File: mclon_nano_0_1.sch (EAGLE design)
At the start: 69 parts, among them J2 10118194-0001LF/C, T1 2N2222, T1.1 BC847, T2 2N2222, T2.1 BC847, U1 TP5400, X1 AK550/2, X2 AK550/2, X3 AK550/2

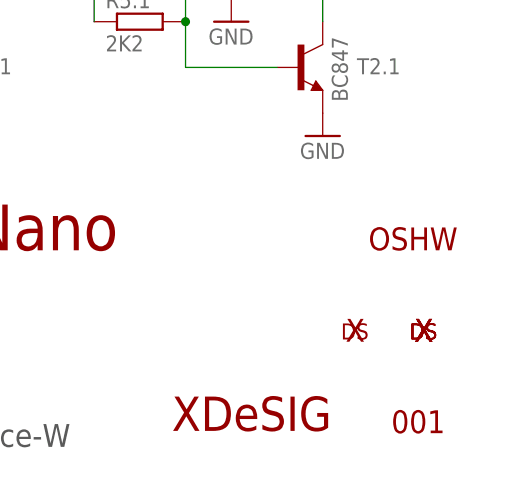
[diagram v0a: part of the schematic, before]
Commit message: Update img
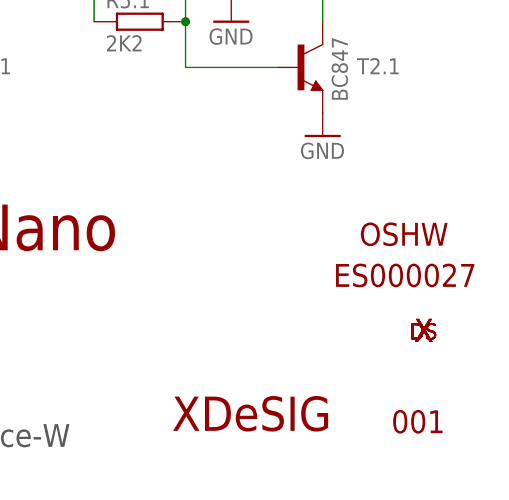
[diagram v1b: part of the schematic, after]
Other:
- note added: "ES000027"
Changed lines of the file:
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@@
 <grid distance="0.1" unitdist="inch" unit="inch" style="lines" multiple="1" display="no" altdistance="0.01" altunitdist="inch" altunit="inch"/>
 <layers>
-<layer number="1" name="Top" color="1" fill="1" visible="yes" active="no"/>
-<layer number="2" name="Route2" color="1" fill="3" visible="yes" active="no"/>
-<layer number="3" name="Route3" color="4" fill="3" visible="yes" active="no"/>
-<layer number="4" name="Route4" color="1" fill="4" visible="yes" active="no"/>
-<layer number="5" name="Route5" color="4" fill="4" visible="yes" active="no"/>
-<layer number="6" name="Route6" color="1" fill="8" visible="yes" active="no"/>
-<layer number="7" name="Route7" color="4" fill="8" visible="yes" active="no"/>
-<layer number="8" name="Route8" color="1" fill="2" visible="yes" active="no"/>
-<layer number="9" name="Route9" color="4" fill="2" visible="yes" active="no"/>
-<layer number="10" name="Route10" color="1" fill="7" visible="yes" active="no"/>
-<layer number="11" name="Route11" color="4" fill="7" visible="yes" active="no"/>
-<layer number="12" name="Route12" color="1" fill="5" visible="yes" active="no"/>
-<layer number="13" name="Route13" color="4" fill="5" visible="yes" active="no"/>
-<layer number="14" name="Route14" color="1" fill="6" visible="yes" active="no"/>
-<layer number="15" name="Route15" color="4" fill="6" visible="yes" active="no"/>
-<layer number="16" name="Bottom" color="4" fill="1" visible="yes" active="no"/>
-<layer number="17" name="Pads" color="2" fill="1" visible="yes" active="no"/>
-<layer number="18" name="Vias" color="2" fill="1" visible="yes" active="no"/>
-<layer number="19" name="Unrouted" color="6" fill="1" visible="yes" active="no"/>
-<layer number="20" name="Dimension" color="24" fill="1" visible="yes" active="no"/>
-<layer number="21" name="tPlace" color="7" fill="1" visible="yes" active="no"/>
-<layer number="22" name="bPlace" color="7" fill="1" visible="yes" active="no"/>
-<layer number="23" name="tOrigins" color="15" fill="1" visible="yes" active="no"/>
-<layer number="24" name="bOrigins" color="15" fill="1" visible="yes" active="no"/>
-<layer number="25" name="tNames" color="7" fill="1" visible="yes" active="no"/>
-<layer number="26" name="bNames" color="7" fill="1" visible="yes" active="no"/>
-<layer number="27" name="tValues" color="7" fill="1" visible="yes" active="no"/>
-<layer number="28" name="bValues" color="7" fill="1" visible="yes" active="no"/>
+<layer number="1" name="Top" color="1" fill="1" visible="no" active="no"/>
+<layer number="2" name="Route2" color="1" fill="3" visible="no" active="no"/>
+<layer number="3" name="Route3" color="4" fill="3" visible="no" active="no"/>
+<layer number="4" name="Route4" color="1" fill="4" visible="no" active="no"/>
+<layer number="5" name="Route5" color="4" fill="4" visible="no" active="no"/>
+<layer number="6" name="Route6" color="1" fill="8" visible="no" active="no"/>
+<layer number="7" name="Route7" color="4" fill="8" visible="no" active="no"/>
+<layer number="8" name="Route8" color="1" fill="2" visible="no" active="no"/>
+<layer number="9" name="Route9" color="4" fill="2" visible="no" active="no"/>
+<layer number="10" name="Route10" color="1" fill="7" visible="no" active="no"/>
+<layer number="11" name="Route11" color="4" fill="7" visible="no" active="no"/>
+<layer number="12" name="Route12" color="1" fill="5" visible="no" active="no"/>
+<layer number="13" name="Route13" color="4" fill="5" visible="no" active="no"/>
+<layer number="14" name="Route14" color="1" fill="6" visible="no" active="no"/>
+<layer number="15" name="Route15" color="4" fill="6" visible="no" active="no"/>
+<layer number="16" name="Bottom" color="4" fill="1" visible="no" active="no"/>
+<layer number="17" name="Pads" color="2" fill="1" visible="no" active="no"/>
+<layer number="18" name="Vias" color="2" fill="1" visible="no" active="no"/>
+<layer number="19" name="Unrouted" color="6" fill="1" visible="no" active="no"/>
+<layer number="20" name="Dimension" color="24" fill="1" visible="no" active="no"/>
+<layer number="21" name="tPlace" color="7" fill="1" visible="no" active="no"/>
+<layer number="22" name="bPlace" color="7" fill="1" visible="no" active="no"/>
+<layer number="23" name="tOrigins" color="15" fill="1" visible="no" active="no"/>
+<layer number="24" name="bOrigins" color="15" fill="1" visible="no" active="no"/>
+<layer number="25" name="tNames" color="7" fill="1" visible="no" active="no"/>
+<layer number="26" name="bNames" color="7" fill="1" visible="no" active="no"/>
+<layer number="27" name="tValues" color="7" fill="1" visible="no" active="no"/>
+<layer number="28" name="bValues" color="7" fill="1" visible="no" active="no"/>
 <layer number="29" name="tStop" color="7" fill="3" visible="no" active="no"/>
 <layer number="30" name="bStop" color="7" fill="6" visible="no" active="no"/>
@@
 <layer number="35" name="tGlue" color="7" fill="4" visible="no" active="no"/>
 <layer number="36" name="bGlue" color="7" fill="5" visible="no" active="no"/>
-<layer number="37" name="tTest" color="7" fill="1" visible="yes" active="no"/>
-<layer number="38" name="bTest" color="7" fill="1" visible="yes" active="no"/>
+<layer number="37" name="tTest" color="7" fill="1" visible="no" active="no"/>
+<layer number="38" name="bTest" color="7" fill="1" visible="no" active="no"/>
 <layer number="39" name="tKeepout" color="4" fill="11" visible="no" active="no"/>
 <layer number="40" name="bKeepout" color="1" fill="11" visible="no" active="no"/>
@@
 <layer number="44" name="Drills" color="7" fill="1" visible="no" active="no"/>
 <layer number="45" name="Holes" color="7" fill="1" visible="no" active="no"/>
-<layer number="46" name="Milling" color="3" fill="1" visible="yes" active="no"/>
-<layer number="47" name="Measures" color="7" fill="1" visible="yes" active="no"/>
-<layer number="48" name="Document" color="7" fill="1" visible="yes" active="no"/>
-<layer number="49" name="Reference" color="7" fill="1" visible="yes" active="no"/>
-<layer number="50" name="dxf" color="7" fill="1" visible="yes" active="no"/>
-<layer number="51" name="tDocu" color="7" fill="1" visible="yes" active="no"/>
-<layer number="52" name="bDocu" color="7" fill="1" visible="yes" active="no"/>
-<layer number="53" name="tGND_GNDA" color="7" fill="9" visible="yes" active="no"/>
-<layer number="54" name="bGND_GNDA" color="1" fill="9" visible="yes" active="no"/>
-<layer number="56" name="wert" color="7" fill="1" visible="yes" active="no"/>
-<layer number="57" name="tCAD" color="7" fill="1" visible="yes" active="no"/>
-<layer number="59" name="tCarbon" color="7" fill="1" visible="yes" active="no"/>
-<layer number="60" name="bCarbon" color="7" fill="1" visible="yes" active="no"/>
+<layer number="46" name="Milling" color="3" fill="1" visible="no" active="no"/>
+<layer number="47" name="Measures" color="7" fill="1" visible="no" active="no"/>
+<layer number="48" name="Document" color="7" fill="1" visible="no" active="no"/>
+<layer number="49" name="Reference" color="7" fill="1" visible="no" active="no"/>
+<layer number="50" name="dxf" color="7" fill="1" visible="no" active="no"/>
+<layer number="51" name="tDocu" color="7" fill="1" visible="no" active="no"/>
+<layer number="52" name="bDocu" color="7" fill="1" visible="no" active="no"/>
+<layer number="53" name="tGND_GNDA" color="7" fill="9" visible="no" active="no"/>
+<layer number="54" name="bGND_GNDA" color="1" fill="9" visible="no" active="no"/>
+<layer number="56" name="wert" color="7" fill="1" visible="no" active="no"/>
+<layer number="57" name="tCAD" color="7" fill="1" visible="no" active="no"/>
+<layer number="59" name="tCarbon" color="7" fill="1" visible="no" active="no"/>
+<layer number="60" name="bCarbon" color="7" fill="1" visible="no" active="no"/>
 <layer number="88" name="SimResults" color="9" fill="1" visible="yes" active="yes"/>
 <layer number="89" name="SimProbes" color="9" fill="1" visible="yes" active="yes"/>
@@
 <text x="51.816" y="56.134" size="5.08" layer="97">Xn THT /  Xn.1 SMD, Choose one</text>
 <text x="72.898" y="39.37" size="1.6764" layer="97">TP5410</text>
+<text x="255.524" y="25.146" size="2.54" layer="94" align="center">ES000027</text>
 </plain>
 <instances>
@@
 </instance>
 <instance part="GND26" gate="1" x="246.38" y="40.64"/>
-<instance part="U$7" gate="G$1" x="256.54" y="27.94"/>
+<instance part="U$7" gate="G$1" x="255.524" y="28.448"/>
 <instance part="D2" gate="G$1" x="115.57" y="18.034" smashed="yes" rot="R90">
 <attribute name="NAME" x="119.253" y="15.24" size="1.778" layer="95" rot="R90"/>
@@
 </instance>
 <instance part="GND28" gate="1" x="144.78" y="8.382"/>
-<instance part="U$8" gate="G$1" x="248.92" y="17.78"/>
+<instance part="U$8" gate="G$1" x="256.54" y="17.78"/>
 </instances>
 <busses>
